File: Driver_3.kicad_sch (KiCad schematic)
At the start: 34 parts

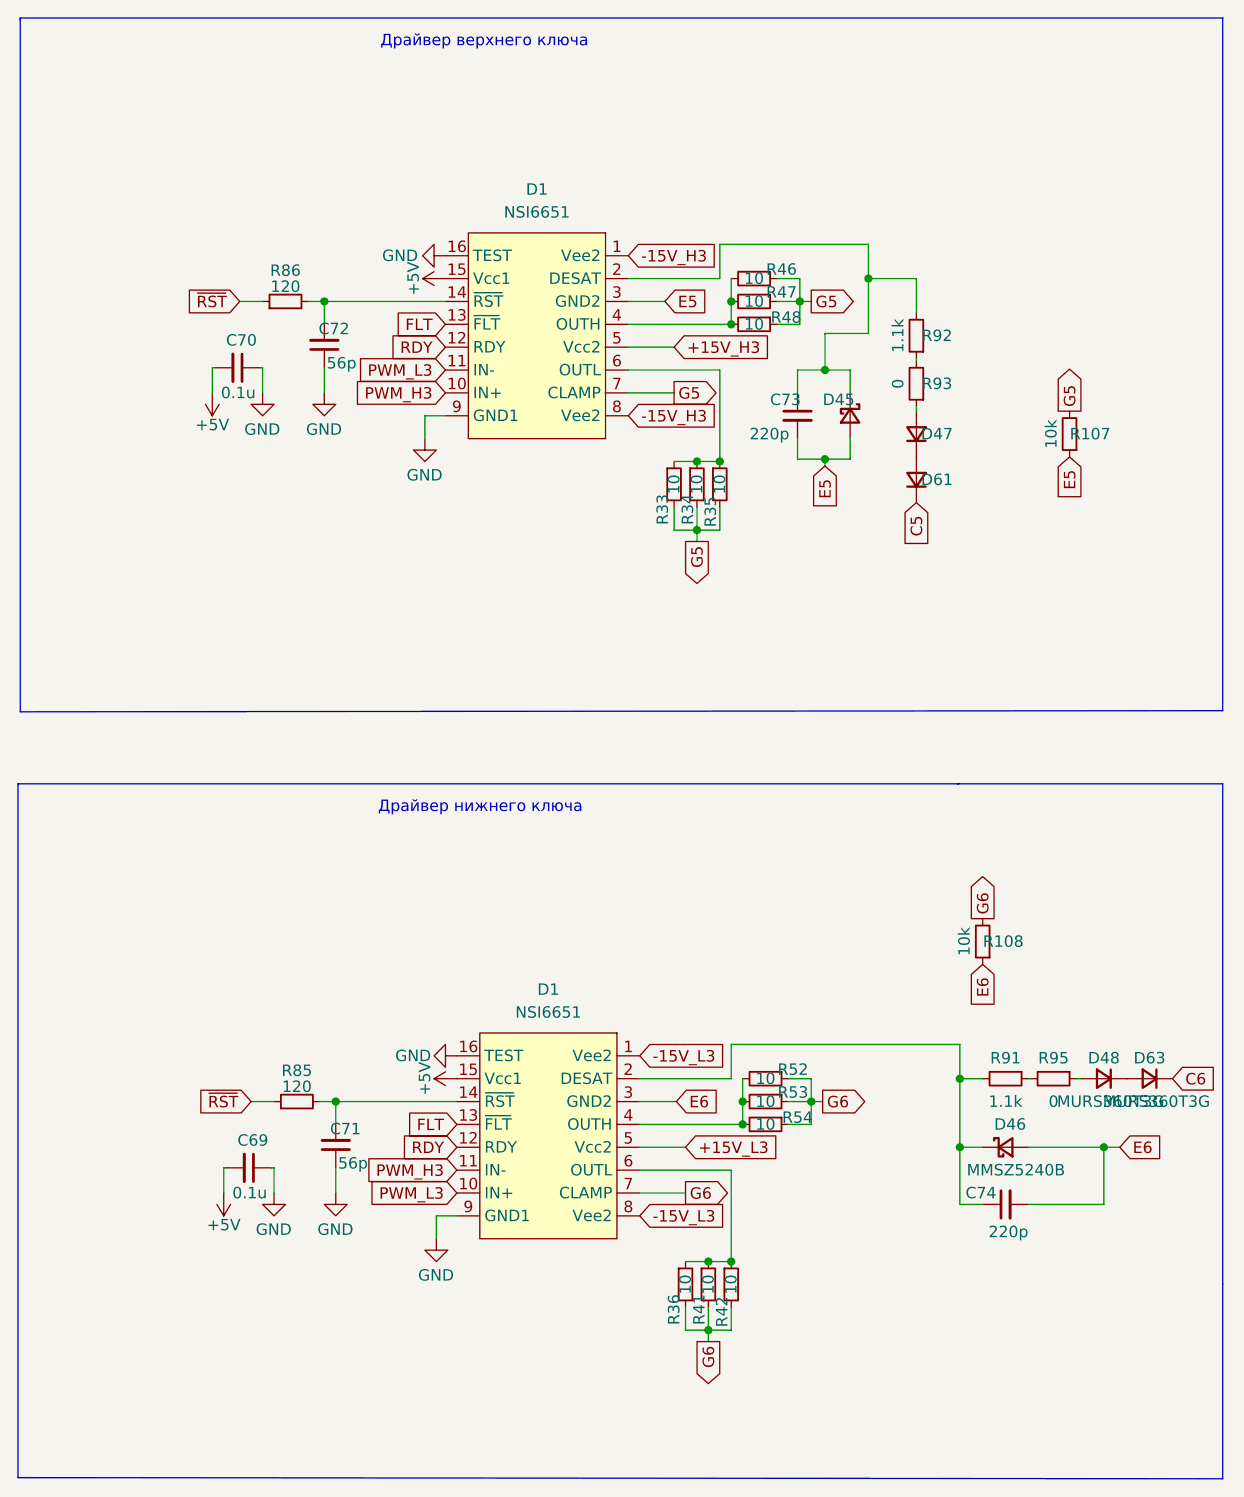
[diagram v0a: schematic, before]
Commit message: Развел вторую стойку
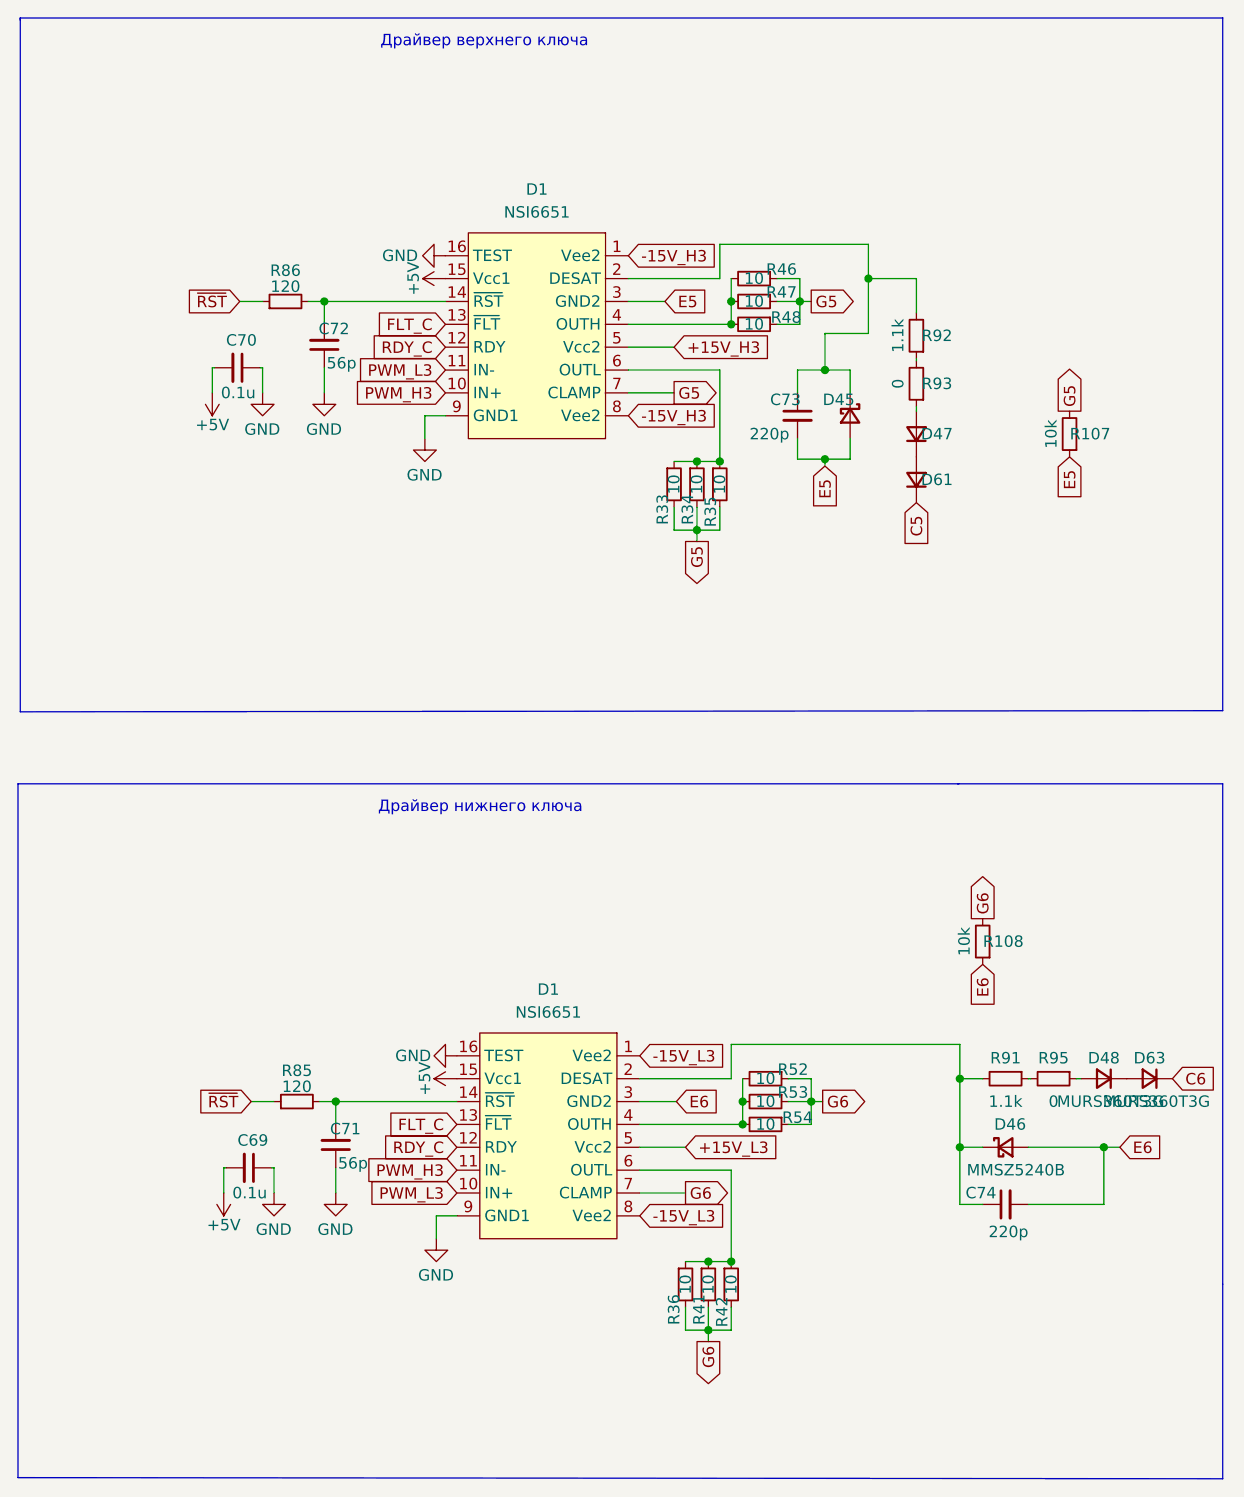
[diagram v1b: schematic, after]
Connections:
- net FLT renamed FLT_C
- net RDY renamed RDY_C
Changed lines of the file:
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@@
 		)
 	)
-	(global_label "RDY"
+	(global_label "RDY_C"
 		(shape input)
 		(at 78.74 59.69 180)
@@
 		)
 		(property "Intersheetrefs" "${INTERSHEET_REFS}"
-			(at 72.7984 59.69 0)
+			(at 69.8886 59.69 0)
 			(effects
 				(font
@@
 		)
 	)
-	(global_label "FLT"
+	(global_label "FLT_C"
 		(shape input)
 		(at 78.74 57.15 180)
@@
 		)
 		(property "Intersheetrefs" "${INTERSHEET_REFS}"
-			(at 73.1806 57.15 0)
+			(at 70.4329 57.15 0)
 			(effects
 				(font
@@
 		)
 	)
-	(global_label "RDY"
+	(global_label "RDY_C"
 		(shape input)
 		(at 80.01 148.59 180)
@@
 		)
 		(property "Intersheetrefs" "${INTERSHEET_REFS}"
-			(at 74.0684 148.59 0)
+			(at 71.1586 148.59 0)
 			(effects
 				(font
@@
 		)
 	)
-	(global_label "FLT"
+	(global_label "FLT_C"
 		(shape input)
 		(at 80.01 146.05 180)
@@
 		)
 		(property "Intersheetrefs" "${INTERSHEET_REFS}"
-			(at 74.4506 146.05 0)
-			(effects
-				(font
+			(at 71.7029 146.05 0)
+			(effects
+				(font
